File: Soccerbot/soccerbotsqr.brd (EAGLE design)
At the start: 127 x 113 mm, 37 parts, among them X1 NXT-SOCKET, X2 NXT-SOCKET, X3 NXT-SOCKET, X4 NXT-SOCKET, X5 NXT-SOCKET, X6 NXT-SOCKET, X7 NXT-SOCKET, X8 NXT-SOCKET

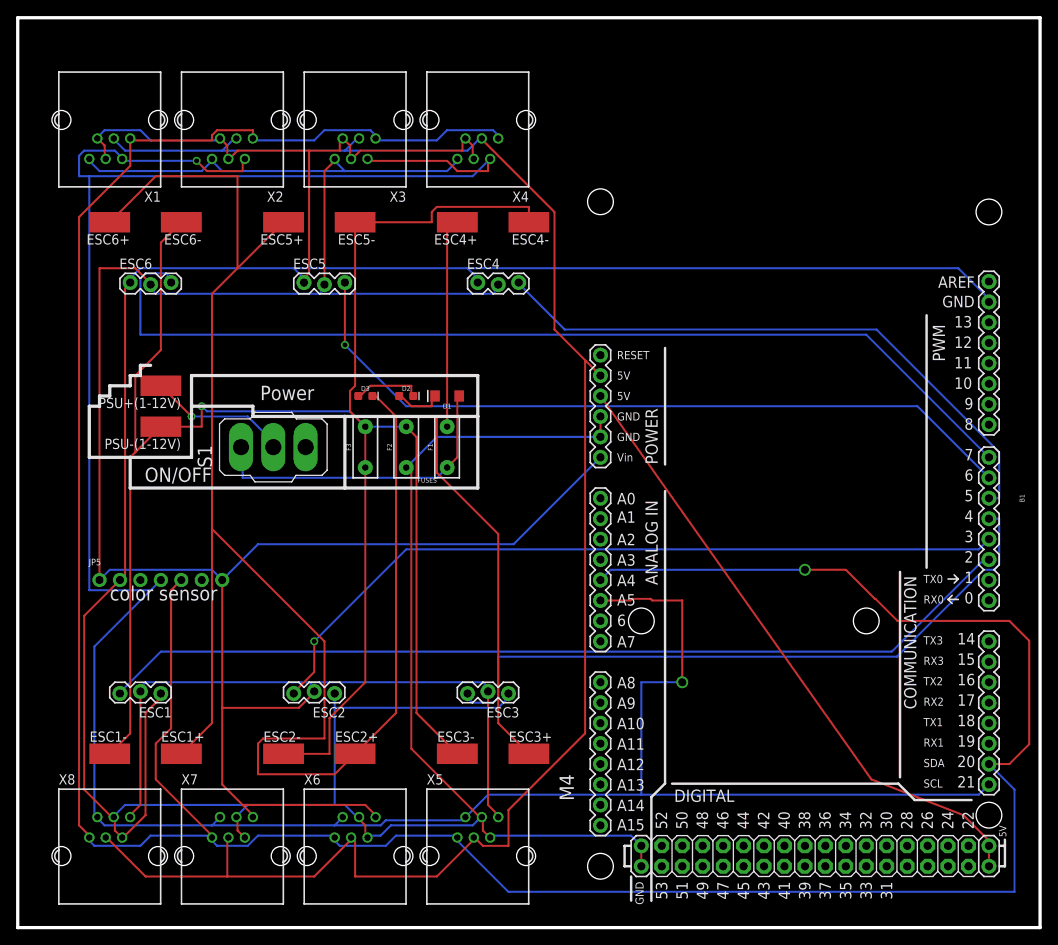
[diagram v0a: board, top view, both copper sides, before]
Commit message: And
And
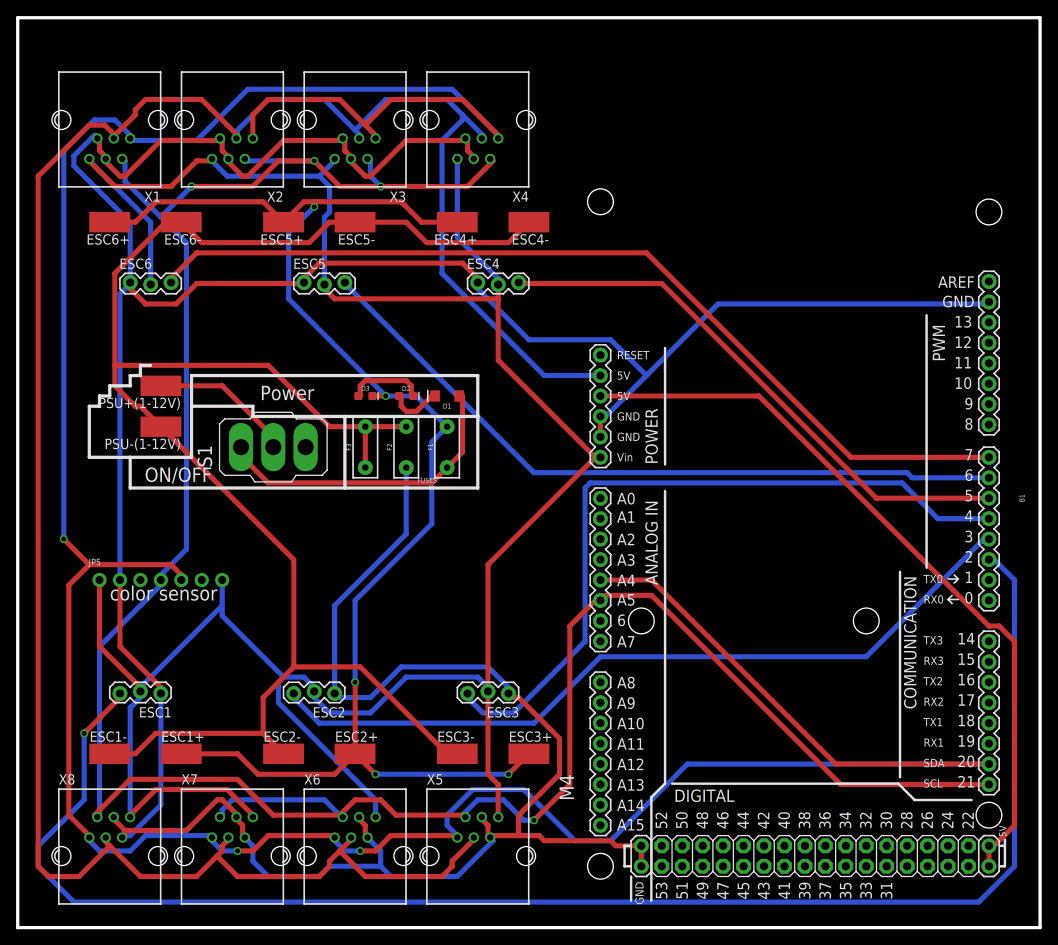
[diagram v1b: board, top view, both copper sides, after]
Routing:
- net BAT+: track 285.2 -> 181.5 mm, vias 0 -> 5
- net D2: track 114.9 -> 190.4 mm, vias 0 -> 1
- net 3.3V: track 217.6 -> 275.8 mm
- net VIN: track 367.5 -> 320.9 mm
- net BAT-: track 251.2 -> 219.5 mm, vias 1 -> 0
- net SCL: track 342.8 -> 319.9 mm, vias 2 -> 4
- net 5.5V: track 78.2 -> 94.0 mm
- net GND: track 476.1 -> 464.7 mm
- net D7: track 123.6 -> 113.9 mm
- net D4: track 83.9 -> 90.9 mm
- net D5: track 75.5 -> 69.6 mm
- net D6: track 94.6 -> 90.1 mm, vias 1 -> 0
- net N$5: track 8.63 -> 9.90 mm
- net D3: track 96.6 -> 97.7 mm, vias 1 -> 0
- net N$3: track 6.25 -> 6.78 mm
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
